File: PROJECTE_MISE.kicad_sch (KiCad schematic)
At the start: 46 parts, among them IC1 MSP430FR2355TPT, J1 conn_DFrobot, J10 SDA_{TP}, J11 SCL_{TP}, J12 SCL_{TP-GND}, J13 SPI_{TP-MISO}, J14 SPI_{TP-SS}, J15 SPI_{TP-SCLK}, J16 SPI_{TP-MOSI}, J17 SPI_{TP-GND}, J2 ESP01_WiFi_mod, J3 Conn_TX_TP, J4 conn_ACLK_{TP}, J5 conn_SMCLK_{TP}, J6 Conn_RX_TP, J8 conn_SBW, J9 SDA_{TP-GND}, SW1 ~{RST_{MSP}}, U1 LMV324, Y2 LFXTAL002997BULK

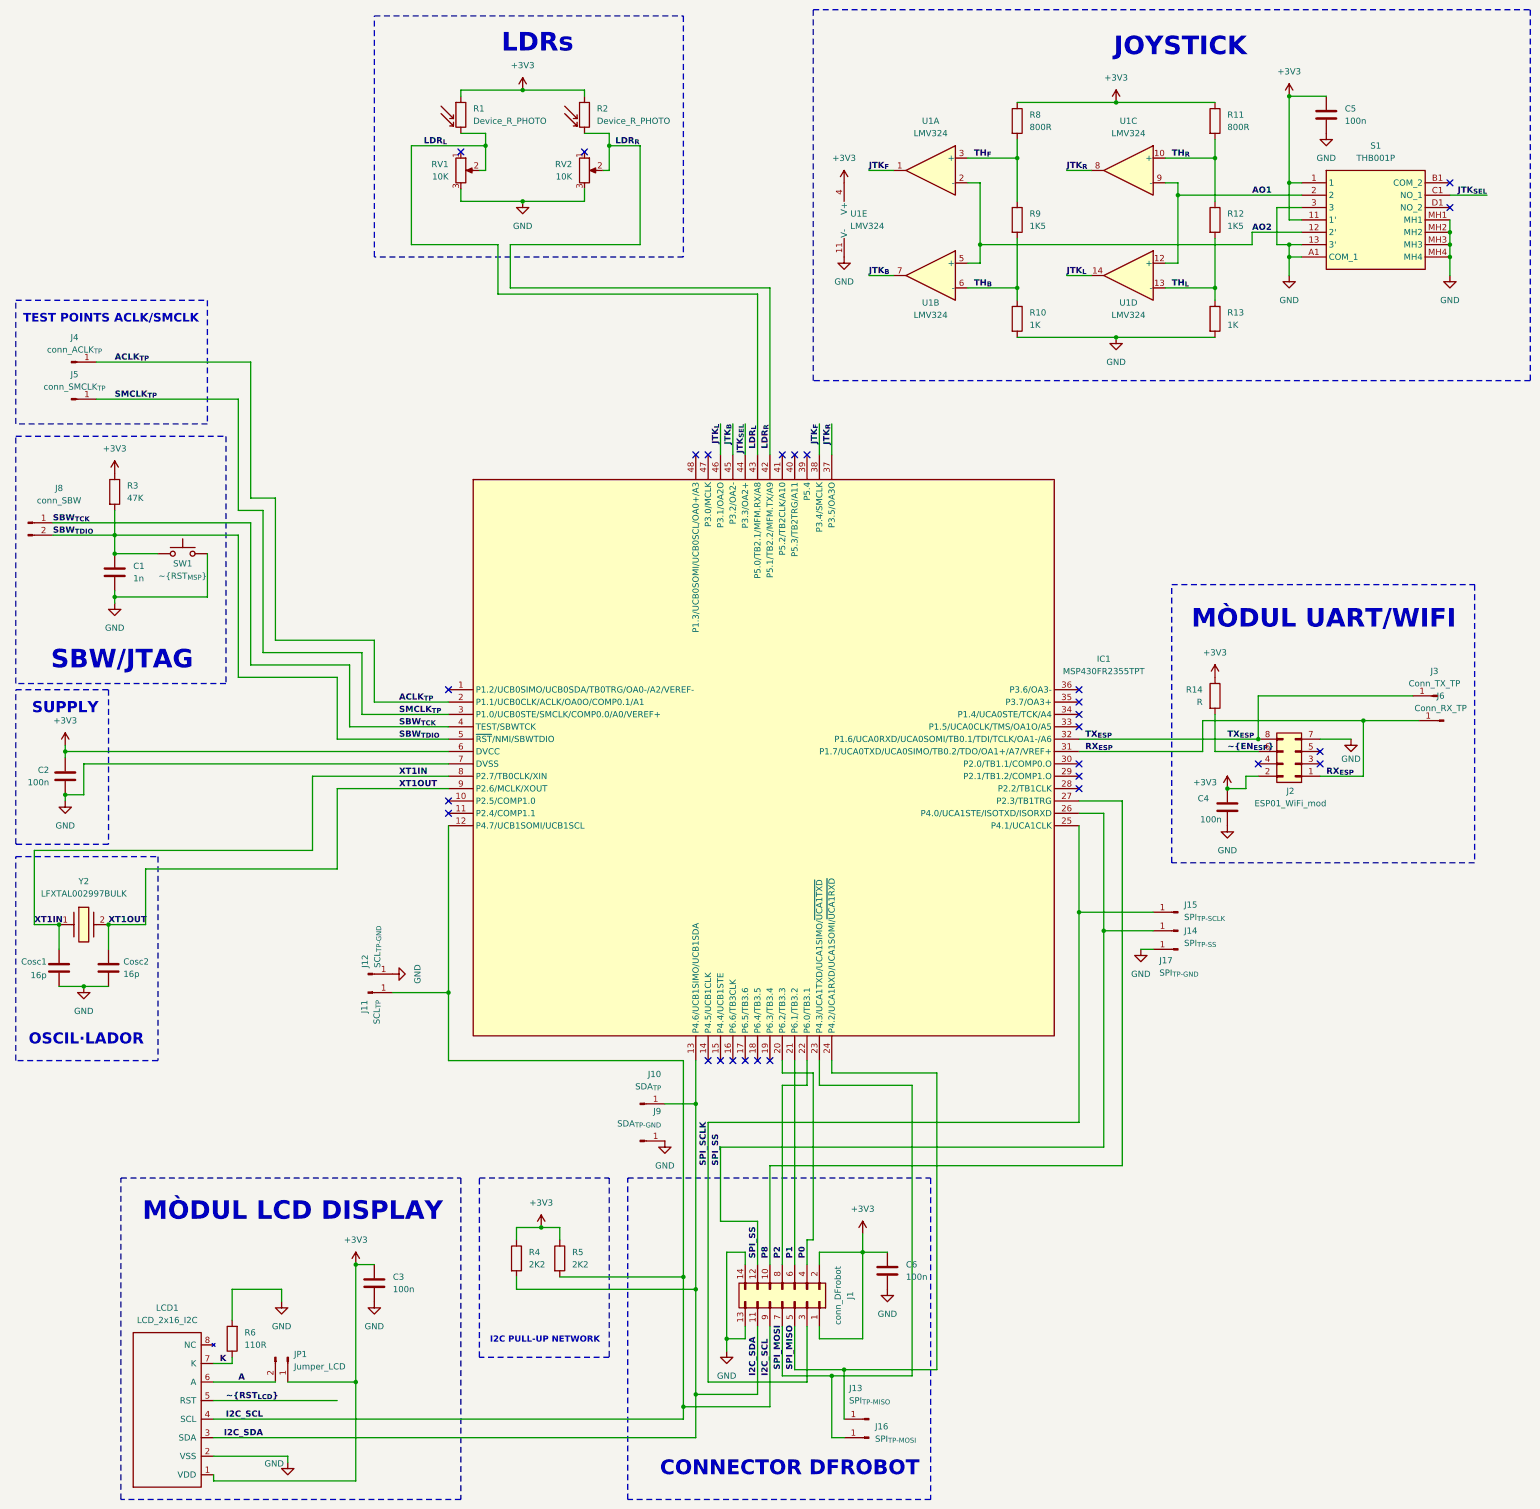
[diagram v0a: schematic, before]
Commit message: layout new placement and nee changes
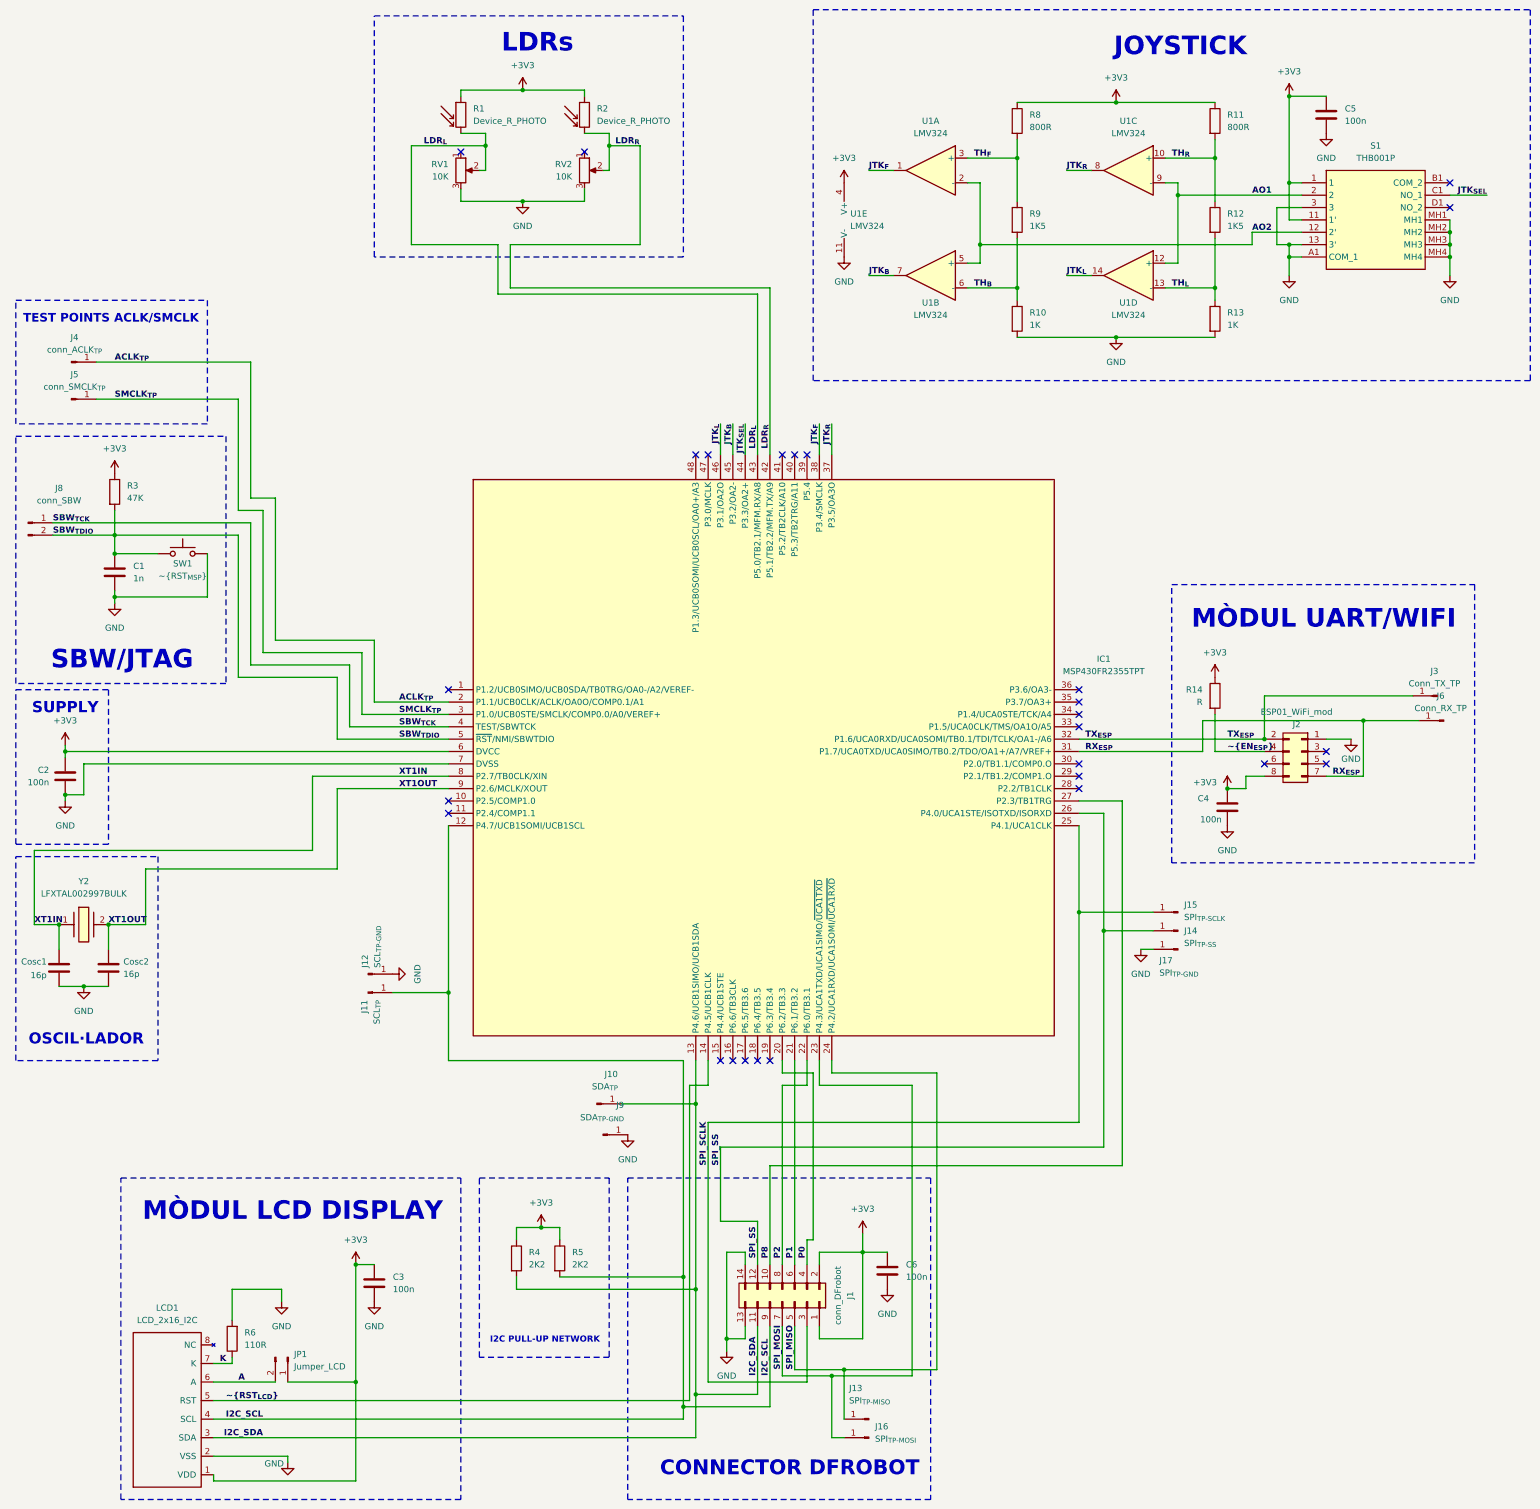
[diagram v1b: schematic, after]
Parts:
- J10, J11, J12, J13, J14, J15, J16, J17, J3, J4, J5, J6, J9: footprint Connector_PinHeader_1.00mm:PinHeader_1x01_P1.00mm_Vertical -> Connector_PinHeader_1.27mm:PinHeader_1x01_P1.27mm_Vertical
- JP1: footprint Connector_PinHeader_1.00mm:PinHeader_1x02_P1.00mm_Vertical -> Connector_PinHeader_1.27mm:PinHeader_2x01_P1.27mm_Vertical
- LCD1: footprint Connector_PinSocket_2.54mm:PinSocket_2x04_P2.54mm_Vertical -> MiSE:LCD_2x16_I2C(Midas)
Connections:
- net +3V3: now also J2.8 (Pin_8); no longer J2.2 (Pin_2)
- net GND: now also J2.1 (Pin_1); no longer J2.7 (Pin_7)
- net RX_{ESP}: now also J2.7 (Pin_7); no longer J2.1 (Pin_1)
- net TX_{ESP}: now also J2.2 (Pin_2); no longer J2.8 (Pin_8)
- net ~{EN_{ESP}}: now also J2.4 (Pin_4); no longer J2.6 (Pin_6)
- net ~{RST_{LCD}}: now also IC1.14 (P4.5/UCB1CLK)
- no-connect marks 28 -> 27
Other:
- moved on the sheet: J10, J2, J9
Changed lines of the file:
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@@
 	)
 	(junction
+		(at 377.19 227.33)
+		(diameter 0)
+		(color 0 0 0 0)
+	)
+	(junction
 		(at 382.27 128.27)
 		(diameter 0)
@@
 	)
 	(junction
-		(at 375.92 227.33)
-		(diameter 0)
-		(color 0 0 0 0)
-	)
-	(junction
 		(at 130.81 238.76)
 		(diameter 0)
@@
 	)
 	(no_connect
-		(at 262.89 293.37)
-	)
-	(no_connect
 		(at 237.49 106.68)
 	)
 	(no_connect
-		(at 388.62 232.41)
+		(at 389.89 232.41)
 	)
 	(no_connect
@@
 	)
 	(no_connect
-		(at 375.92 232.41)
+		(at 377.19 232.41)
 	)
 	(no_connect
@@
 	)
 	(no_connect
-		(at 388.62 229.87)
+		(at 389.89 229.87)
 	)
 	(no_connect
@@
 	(wire
 		(pts
-			(xy 388.62 234.95) (xy 397.51 234.95)
+			(xy 339.09 229.87) (xy 364.49 229.87)
 		)
 		(stroke
@@
 	(wire
 		(pts
-			(xy 339.09 229.87) (xy 364.49 229.87)
+			(xy 389.89 234.95) (xy 397.51 234.95)
 		)
 		(stroke
@@
 	(wire
 		(pts
-			(xy 367.03 229.87) (xy 375.92 229.87)
+			(xy 367.03 229.87) (xy 377.19 229.87)
 		)
 		(stroke
@@
 	(wire
 		(pts
+			(xy 259.08 363.22) (xy 259.08 298.45)
+		)
+		(stroke
+			(width 0)
+			(type default)
+		)
+	)
+	(wire
+		(pts
 			(xy 165.1 355.6) (xy 165.1 354.33)
 		)
@@
 	(wire
 		(pts
-			(xy 373.38 234.95) (xy 375.92 234.95)
+			(xy 373.38 234.95) (xy 377.19 234.95)
 		)
 		(stroke
@@
 	(wire
 		(pts
+			(xy 377.19 218.44) (xy 377.19 227.33)
+		)
+		(stroke
+			(width 0)
+			(type default)
+		)
+	)
+	(wire
+		(pts
 			(xy 166.37 214.63) (xy 186.69 214.63)
 		)
@@
 	(wire
 		(pts
-			(xy 339.09 227.33) (xy 375.92 227.33)
+			(xy 339.09 227.33) (xy 377.19 227.33)
 		)
 		(stroke
@@
 	(wire
 		(pts
-			(xy 388.62 227.33) (xy 394.97 227.33)
+			(xy 389.89 227.33) (xy 394.97 227.33)
 		)
 		(stroke
@@
 	(wire
 		(pts
-			(xy 375.92 218.44) (xy 407.67 218.44)
+			(xy 377.19 218.44) (xy 407.67 218.44)
 		)
 		(stroke
@@
 	(wire
 		(pts
-			(xy 290.83 370.84) (xy 288.29 370.84)
+			(xy 262.89 293.37) (xy 262.89 298.45)
 		)
 		(stroke
@@
 	(wire
 		(pts
-			(xy 288.29 370.84) (xy 288.29 358.14)
+			(xy 290.83 370.84) (xy 288.29 370.84)
 		)
 		(stroke
@@
 	(wire
 		(pts
-			(xy 186.69 227.33) (xy 209.55 227.33)
+			(xy 288.29 370.84) (xy 288.29 358.14)
 		)
 		(stroke
@@
 	(wire
 		(pts
-			(xy 375.92 227.33) (xy 375.92 218.44)
+			(xy 186.69 227.33) (xy 209.55 227.33)
 		)
 		(stroke
@@
 	(wire
 		(pts
-			(xy 254 302.26) (xy 260.35 302.26)
+			(xy 245.11 302.26) (xy 260.35 302.26)
+		)
+		(stroke
+			(width 0)
+			(type default)
+		)
+	)
+	(wire
+		(pts
+			(xy 259.08 298.45) (xy 262.89 298.45)
 		)
 		(stroke
@@
 	(wire
 		(pts
-			(xy 161.29 363.22) (xy 186.69 363.22)
+			(xy 161.29 363.22) (xy 259.08 363.22)
 		)
 		(stroke
@@
 	)
 	(label "RX_{ESP}"
-		(at 389.89 234.95 0)
+		(at 391.16 234.95 0)
 		(effects
 			(font
@@
 	(symbol
 		(lib_id "power:GND")
-		(at 254 309.88 0)
+		(at 246.38 308.61 0)
 		(unit 1)
 		(exclude_from_sim no)
@@
 		(fields_autoplaced yes)
 		(property "Reference" "#PWR28"
-			(at 254 316.23 0)
+			(at 246.38 314.96 0)
 			(effects
 				(font
@@
 		)
 		(property "Value" "GND"
-			(at 254 314.96 0)
+			(at 246.38 313.69 0)
 			(effects
 				(font
@@
 		)
 		(property "Footprint" ""
-			(at 254 309.88 0)
+			(at 246.38 308.61 0)
 			(effects
 				(font
@@
 		)
 		(property "Datasheet" ""
-			(at 254 309.88 0)
+			(at 246.38 308.61 0)
 			(effects
 				(font
@@
 		)
 		(property "Description" "Power symbol creates a global label with name \"GND\" , ground"
-			(at 254 309.88 0)
+			(at 246.38 308.61 0)
 			(effects
 				(font
@@
 	(symbol
 		(lib_id "Connector_Generic:Conn_02x04_Odd_Even")
-		(at 383.54 232.41 180)
+		(at 384.81 229.87 0)
+		(mirror y)
 		(unit 1)
 		(exclude_from_sim no)
@@
 		(dnp no)
 		(property "Reference" "J2"
-			(at 382.524 237.998 0)
+			(at 383.794 224.282 0)
 			(effects
 				(font
@@
 		)
 		(property "Value" "ESP01_WiFi_mod"
-			(at 382.524 240.538 0)
+			(at 383.794 221.742 0)
 			(effects
 				(font
@@
 		)
 		(property "Footprint" "Connector_PinSocket_2.54mm:PinSocket_2x04_P2.54mm_Vertical"
-			(at 383.54 232.41 0)
+			(at 384.81 229.87 0)
 			(effects
 				(font
@@
 		)
 		(property "Datasheet" "~"
-			(at 383.54 232.41 0)
+			(at 384.81 229.87 0)
 			(effects
 				(font
@@
 		)
 		(property "Description" "Generic connector, double row, 02x04, odd/even pin numbering scheme (row 1 odd numbers, row 2 even numbers), script generated (kicad-library-utils/schlib/autogen/connector/)"
-			(at 383.54 232.41 0)
+			(at 384.81 229.87 0)
 			(effects
 				(font
@@
 			)
 		)
-		(property "Footprint" "Connector_PinHeader_1.00mm:PinHeader_1x01_P1.00mm_Vertical"
+		(property "Footprint" "Connector_PinHeader_1.27mm:PinHeader_1x01_P1.27mm_Vertical"
 			(at 359.41 270.51 0)
 			(effects
@@
 			)
 		)
-		(property "Footprint" "Connector_PinHeader_1.00mm:PinHeader_1x01_P1.00mm_Vertical"
+		(property "Footprint" "Connector_PinHeader_1.27mm:PinHeader_1x01_P1.27mm_Vertical"
 			(at 193.04 275.59 0)
 			(effects
@@
 	(symbol
 		(lib_id "Connector:Conn_01x01_Pin")
-		(at 248.92 309.88 0)
+		(at 241.3 308.61 0)
 		(unit 1)
 		(exclude_from_sim no)
@@
 		(dnp no)
 		(property "Reference" "J9"
-			(at 253.238 303.784 0)
+			(at 245.618 302.514 0)
 			(effects
 				(font
@@
 		)
 		(property "Value" "SDA_{TP-GND}"
-			(at 253.238 306.324 0)
+			(at 245.618 305.054 0)
 			(effects
 				(font
@@
 			)
 		)
-		(property "Footprint" "Connector_PinHeader_1.00mm:PinHeader_1x01_P1.00mm_Vertical"
-			(at 248.92 309.88 0)
+		(property "Footprint" "Connector_PinHeader_1.27mm:PinHeader_1x01_P1.27mm_Vertical"
+			(at 241.3 308.61 0)
 			(effects
 				(font
@@
 		)
 		(property "Datasheet" "~"
-			(at 248.92 309.88 0)
+			(at 241.3 308.61 0)
 			(effects
 				(font
@@
 		)
 		(property "Description" "Generic connector, single row, 01x01, script generated"
-			(at 248.92 309.88 0)
+			(at 241.3 308.61 0)
 			(effects
 				(font
@@
 			)
 		)
-		(property "Footprint" "Connector_PinHeader_1.00mm:PinHeader_1x01_P1.00mm_Vertical"
+		(property "Footprint" "Connector_PinHeader_1.27mm:PinHeader_1x01_P1.27mm_Vertical"
 			(at 359.41 266.7 0)
 			(effects
@@
 			)
 		)
-		(property "Footprint" "Connector_PinHeader_1.00mm:PinHeader_1x01_P1.00mm_Vertical"
+		(property "Footprint" "Connector_PinHeader_1.27mm:PinHeader_1x01_P1.27mm_Vertical"
 			(at 295.91 370.84 0)
 			(effects
@@
 			)
 		)
-		(property "Footprint" "Connector_PinHeader_1.00mm:PinHeader_1x01_P1.00mm_Vertical"
+		(property "Footprint" "Connector_PinHeader_1.27mm:PinHeader_1x01_P1.27mm_Vertical"
 			(at 414.02 223.52 0)
 			(effects
@@
 	(symbol
 		(lib_id "Connector:Conn_01x01_Pin")
-		(at 248.92 302.26 0)
+		(at 240.03 302.26 0)
 		(unit 1)
 		(exclude_from_sim no)
@@
 		(dnp no)
 		(property "Reference" "J10"
-			(at 253.238 296.164 0)
+			(at 244.348 296.164 0)
 			(effects
 				(font
@@
 		)
 		(property "Value" "SDA_{TP}"
-			(at 253.238 298.704 0)
+			(at 244.348 298.704 0)
 			(effects
 				(font
@@
 			)
 		)
-		(property "Footprint" "Connector_PinHeader_1.00mm:PinHeader_1x01_P1.00mm_Vertical"
-			(at 248.92 302.26 0)
+		(property "Footprint" "Connector_PinHeader_1.27mm:PinHeader_1x01_P1.27mm_Vertical"
+			(at 240.03 302.26 0)
 			(effects
 				(font
@@
 		)
 		(property "Datasheet" "~"
-			(at 248.92 302.26 0)
+			(at 240.03 302.26 0)
 			(effects
 				(font
@@
 		)
 		(property "Description" "Generic connector, single row, 01x01, script generated"
-			(at 248.92 302.26 0)
+			(at 240.03 302.26 0)
 			(effects
 				(font
@@
 			)
 		)
-		(property "Footprint" "Connector_PinSocket_2.54mm:PinSocket_2x04_P2.54mm_Vertical"
+		(property "Footprint" "MiSE:LCD_2x16_I2C(Midas)"
 			(at 138.43 368.3 0)
 			(effects
@@
 			)
 		)
-		(property "Footprint" "Connector_PinHeader_1.00mm:PinHeader_1x01_P1.00mm_Vertical"
+		(property "Footprint" "Connector_PinHeader_1.27mm:PinHeader_1x01_P1.27mm_Vertical"
 			(at 193.04 279.4 0)
 			(effects
@@
 			)
 		)
-		(property "Footprint" "Connector_PinHeader_1.00mm:PinHeader_1x01_P1.00mm_Vertical"
+		(property "Footprint" "Connector_PinHeader_1.27mm:PinHeader_1x01_P1.27mm_Vertical"
 			(at 359.41 262.89 0)
 			(effects
@@
 			)
 		)
-		(property "Footprint" "Connector_PinHeader_1.00mm:PinHeader_1x01_P1.00mm_Vertical"
+		(property "Footprint" "Connector_PinHeader_1.27mm:PinHeader_1x01_P1.27mm_Vertical"
 			(at 132.08 149.86 0)
 			(effects
@@
 			)
 		)
-		(property "Footprint" "Connector_PinHeader_1.00mm:PinHeader_1x01_P1.00mm_Vertical"
+		(property "Footprint" "Connector_PinHeader_1.27mm:PinHeader_1x01_P1.27mm_Vertical"
 			(at 412.75 218.44 0)
 			(effects
@@
 			)
 		)
-		(property "Footprint" "Connector_PinHeader_1.00mm:PinHeader_1x02_P1.00mm_Vertical"
+		(property "Footprint" "Connector_PinHeader_1.27mm:PinHeader_2x01_P1.27mm_Vertical"
 			(at 176.53 354.33 0)
 			(effects
@@
 			)
 		)
-		(property "Footprint" "Connector_PinHeader_1.00mm:PinHeader_1x01_P1.00mm_Vertical"
+		(property "Footprint" "Connector_PinHeader_1.27mm:PinHeader_1x01_P1.27mm_Vertical"
 			(at 132.08 157.48 0)
 			(effects
@@
 			)
 		)
-		(property "Footprint" "Connector_PinHeader_1.00mm:PinHeader_1x01_P1.00mm_Vertical"
+		(property "Footprint" "Connector_PinHeader_1.27mm:PinHeader_1x01_P1.27mm_Vertical"
 			(at 295.91 367.03 0)
 			(effects
